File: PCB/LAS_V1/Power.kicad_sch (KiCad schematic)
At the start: 6 parts, among them U2 XL1509-5.0

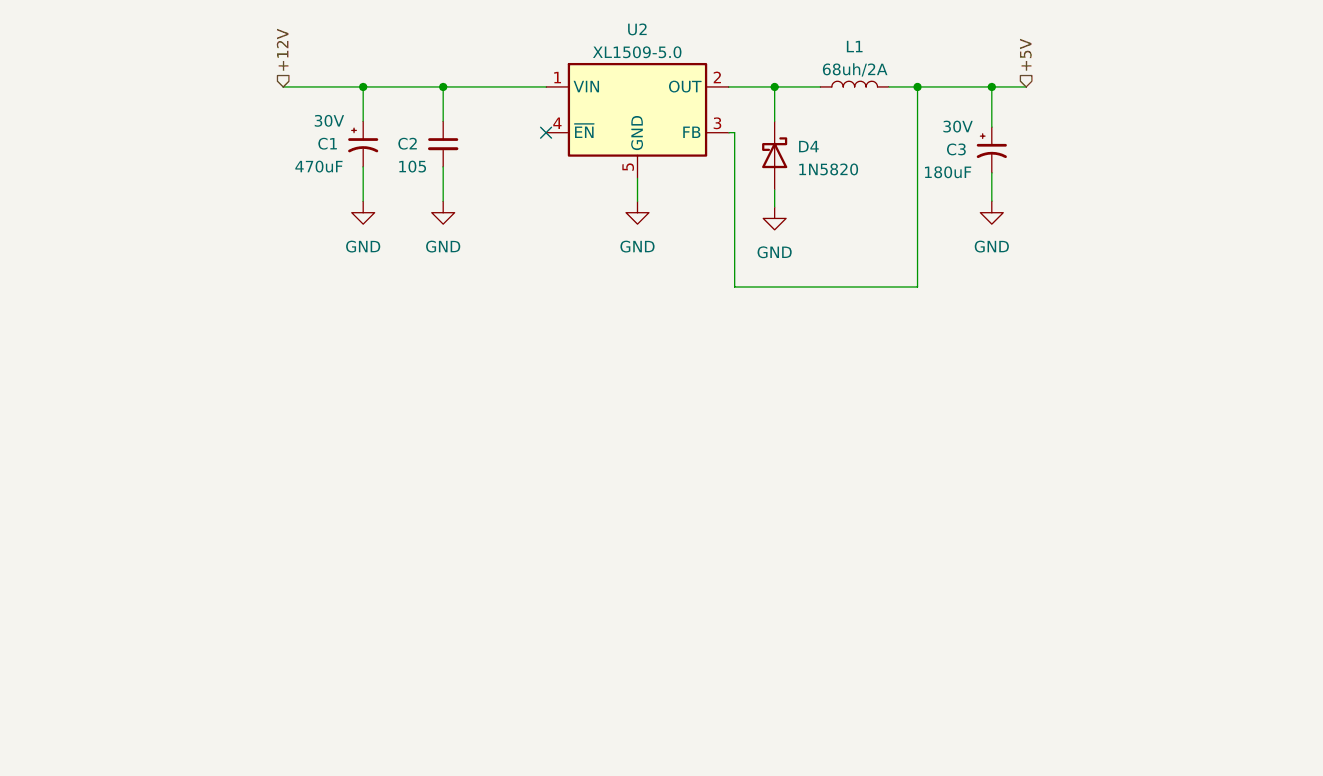
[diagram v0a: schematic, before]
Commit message: -am
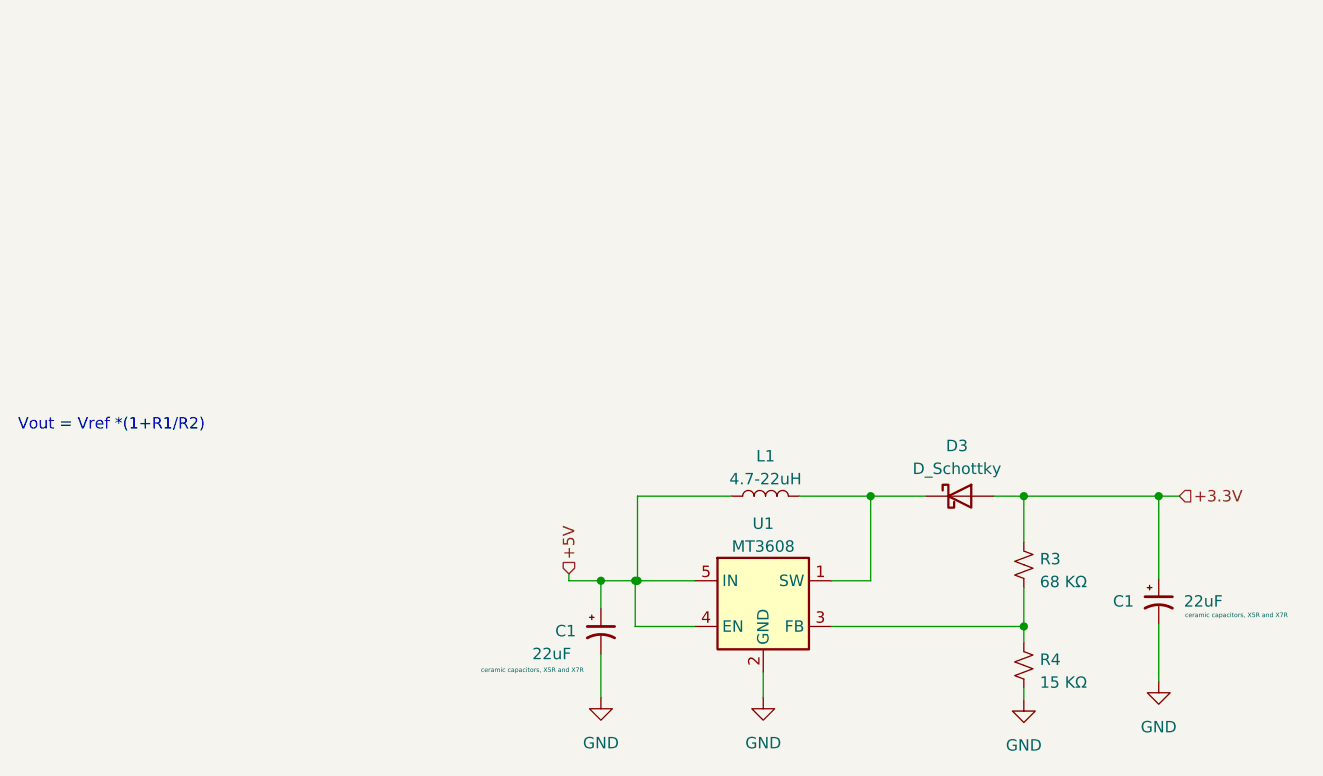
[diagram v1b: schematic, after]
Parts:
- removed C1: 470uF, symbol Device:C_Polarized_Small_US
- removed C2: 105, symbol Device:C_Small
- removed C3: 180uF, symbol Device:C_Polarized_Small_US
- removed D4: 1N5820, Diode_THT:D_DO-201AD_P15.24mm_Horizontal, symbol Diode:1N5820
- removed U2: XL1509-5.0, Package_SO:SOIC-8_3.9x4.9mm_P1.27mm, symbol Regulator_Switching:XL1509-5.0
- added C1 (x2): 22uF, symbol Device:C_Polarized_Small_US
- added D3: D_Schottky, symbol Device:D_Schottky
- added R3: 68 KΩ, symbol Device:R_Small_US
- added R4: 15 KΩ, symbol Device:R_Small_US
- added U1: MT3608, Package_TO_SOT_SMD:SOT-23-6, symbol Regulator_Switching:MT3608
- L1: value 68uh/2A -> 4.7-22uH
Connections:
- net +5V: now also L1.1, C1.1, U1.4 (EN), U1.5 (IN); no longer L1.2
- net GND: now also C1.2, C1.2, R4.2, U1.2 (GND)
- new net: D3.1 (K), L1.2, U1.1 (SW)
- new net: R3.2, R4.1, U1.3 (FB)
- new net +3.3V: C1.1, D3.2 (A), R3.1
- no-connect marks 1 -> 0
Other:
- note added: "Vout = Vref *(1+R1/R2)"

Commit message: installing JLB, PCB mostly done
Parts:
- removed C1 (x2): 22uF, symbol Device:C_Polarized_Small_US
- removed D3: D_Schottky, symbol Device:D_Schottky
- removed L1: 4.7-22uH, symbol Device:L
- removed R3: 68 KΩ, symbol Device:R_Small_US
- removed R4: 15 KΩ, symbol Device:R_Small_US
- removed U1: MT3608, Package_TO_SOT_SMD:SOT-23-6, symbol Regulator_Switching:MT3608
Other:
- note removed: "Vout = Vref *(1+R1/R2)"
